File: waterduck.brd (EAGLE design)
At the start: 72.4 x 60.6 mm, 11 parts, among them U1 FEATHER, U2 ATLAS-DO, U3 ATLAS-PH, X1 5268-02, X2 5268-03, X3 5268-02, X4 5268-02

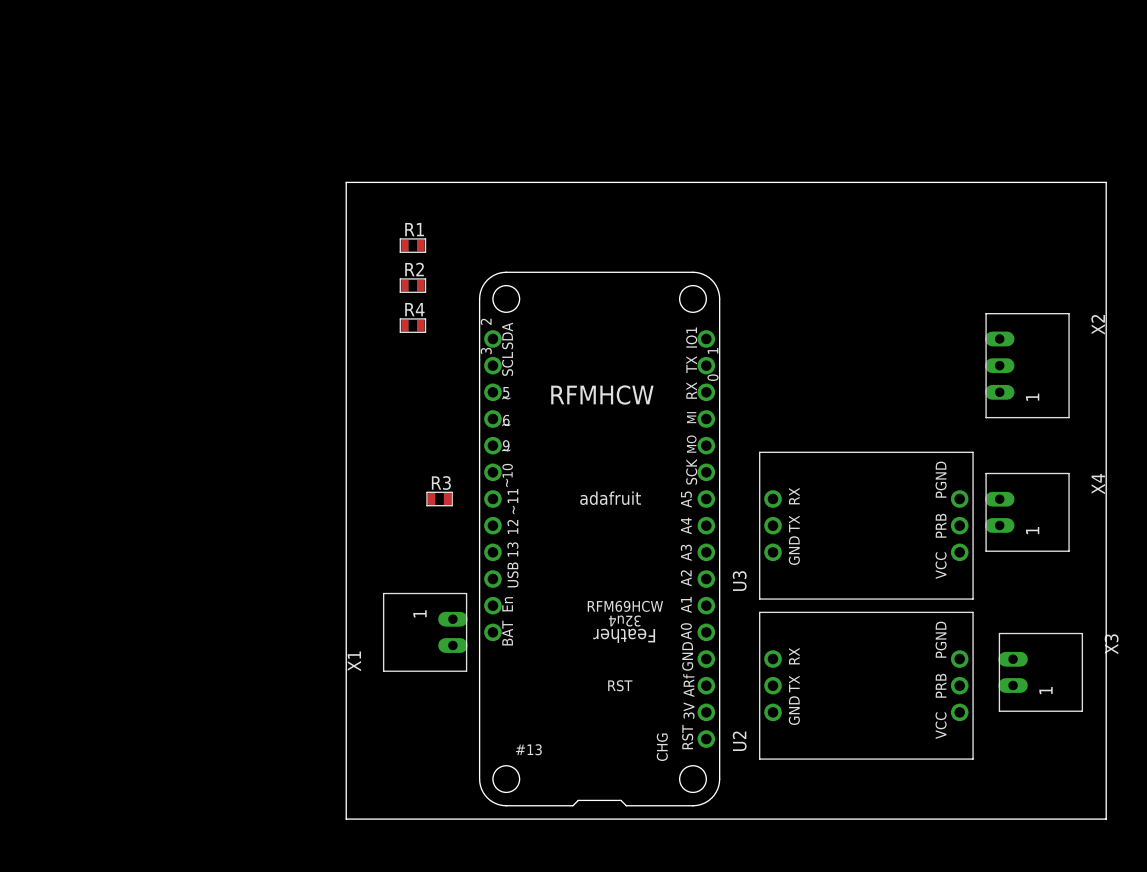
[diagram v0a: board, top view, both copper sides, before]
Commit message: gerber
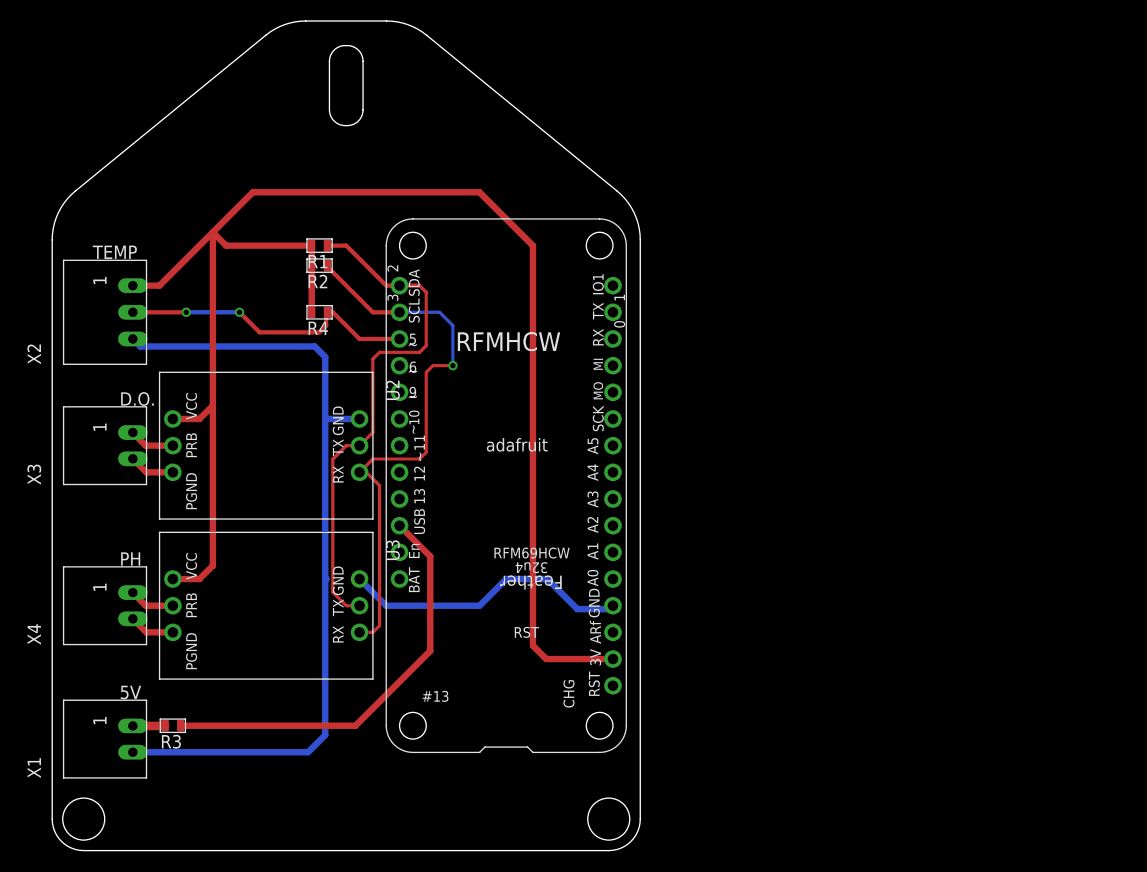
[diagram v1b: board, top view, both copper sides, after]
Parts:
- moved X3 86.6 mm to (-20.3, 35.6), turned to 90 degrees
- moved X4 83.0 mm to (-20.3, 20.3), turned to 90 degrees
- moved X2 82.7 mm to (-20.3, 48.3), turned to 90 degrees
- moved U2 80.8 mm to (-17.8, 35.6), turned to 270 degrees
- moved U3 77.8 mm to (-17.8, 20.3), turned to 270 degrees
- moved R3 33.3 mm to (-16.5, 8.89), turned to 180 degrees
- moved X1 32.1 mm to (-20.3, 7.62)
- moved U1 10.2 mm to (26.7, 6.35)
- moved R2 9.09 mm to (-2.54, 52.7), turned to 180 degrees
- moved R4 8.98 mm to (-2.54, 48.3), turned to 180 degrees
- moved R1 8.89 mm to (-2.54, 54.6), turned to 180 degrees
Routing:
- net +3V3: track 0.00 -> 146.8 mm
- net GND: track 0.00 -> 105.1 mm
- net SCL: track 0.00 -> 53.7 mm, vias 0 -> 1
- net SDA: track 0.00 -> 49.6 mm
- net VBUS: track 0.00 -> 39.9 mm
- net TEMP: track 0.00 -> 28.7 mm, vias 0 -> 2
- net N$4: track 0.00 -> 4.34 mm
- net N$2: track 0.00 -> 4.34 mm
- net N$3: track 0.00 -> 4.33 mm
- net N$1: track 0.00 -> 4.33 mm
- net N$5: track 0.00 -> 3.08 mm
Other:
- board size 72.4 x 60.6 mm -> 56 x 79 mm
- board text added: "5V"
- board text added: "D.O."
- board text added: "PH"
- board text added: "TEMP"
